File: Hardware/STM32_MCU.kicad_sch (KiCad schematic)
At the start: 1 part, among them U1 STM32G431RBTx

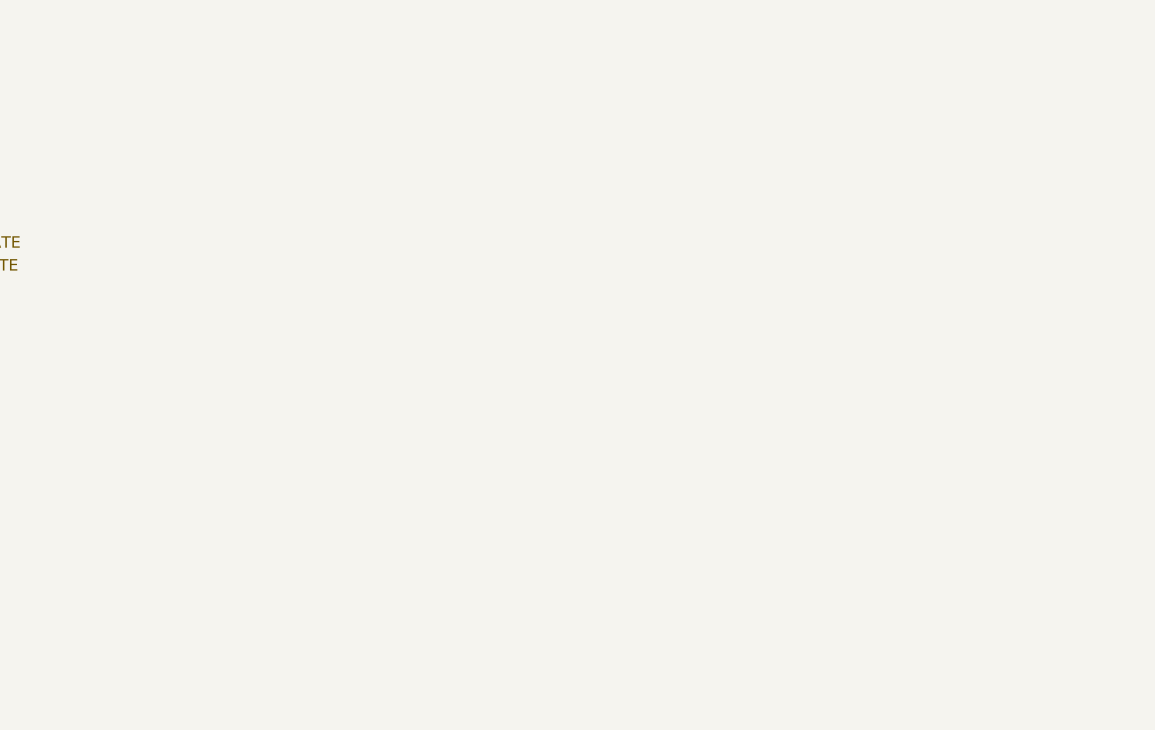
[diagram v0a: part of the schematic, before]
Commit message: Set footprint + excludes
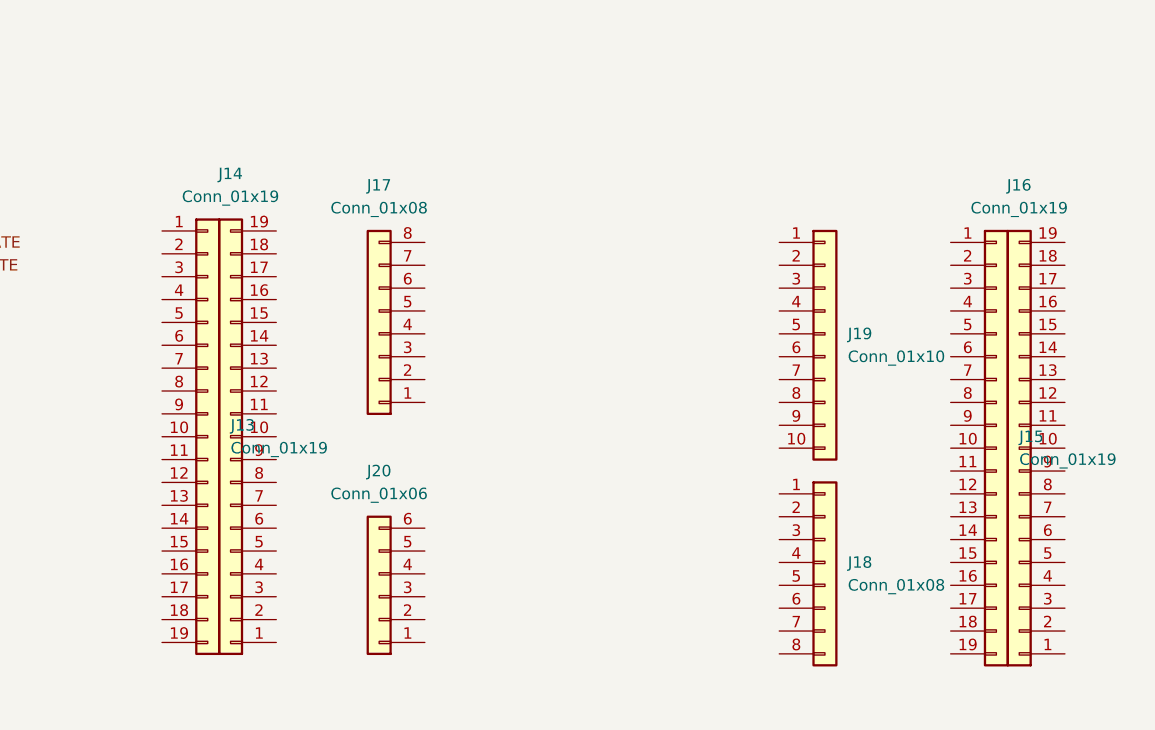
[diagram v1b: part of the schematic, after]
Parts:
- added J13, J14, J15, J16: Conn_01x19, symbol Connector_Generic:Conn_01x19
- added J17, J18: Conn_01x08, symbol Connector_Generic:Conn_01x08
- added J19: Conn_01x10, symbol Connector_Generic:Conn_01x10
- added J20: Conn_01x06, symbol Connector_Generic:Conn_01x06
- U1: now left out of the parts list
